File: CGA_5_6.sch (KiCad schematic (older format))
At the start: 5 parts, among them U13 74LS08, U15 74LS00, U20 74LS04, U21 74LS174, U64 74LS164

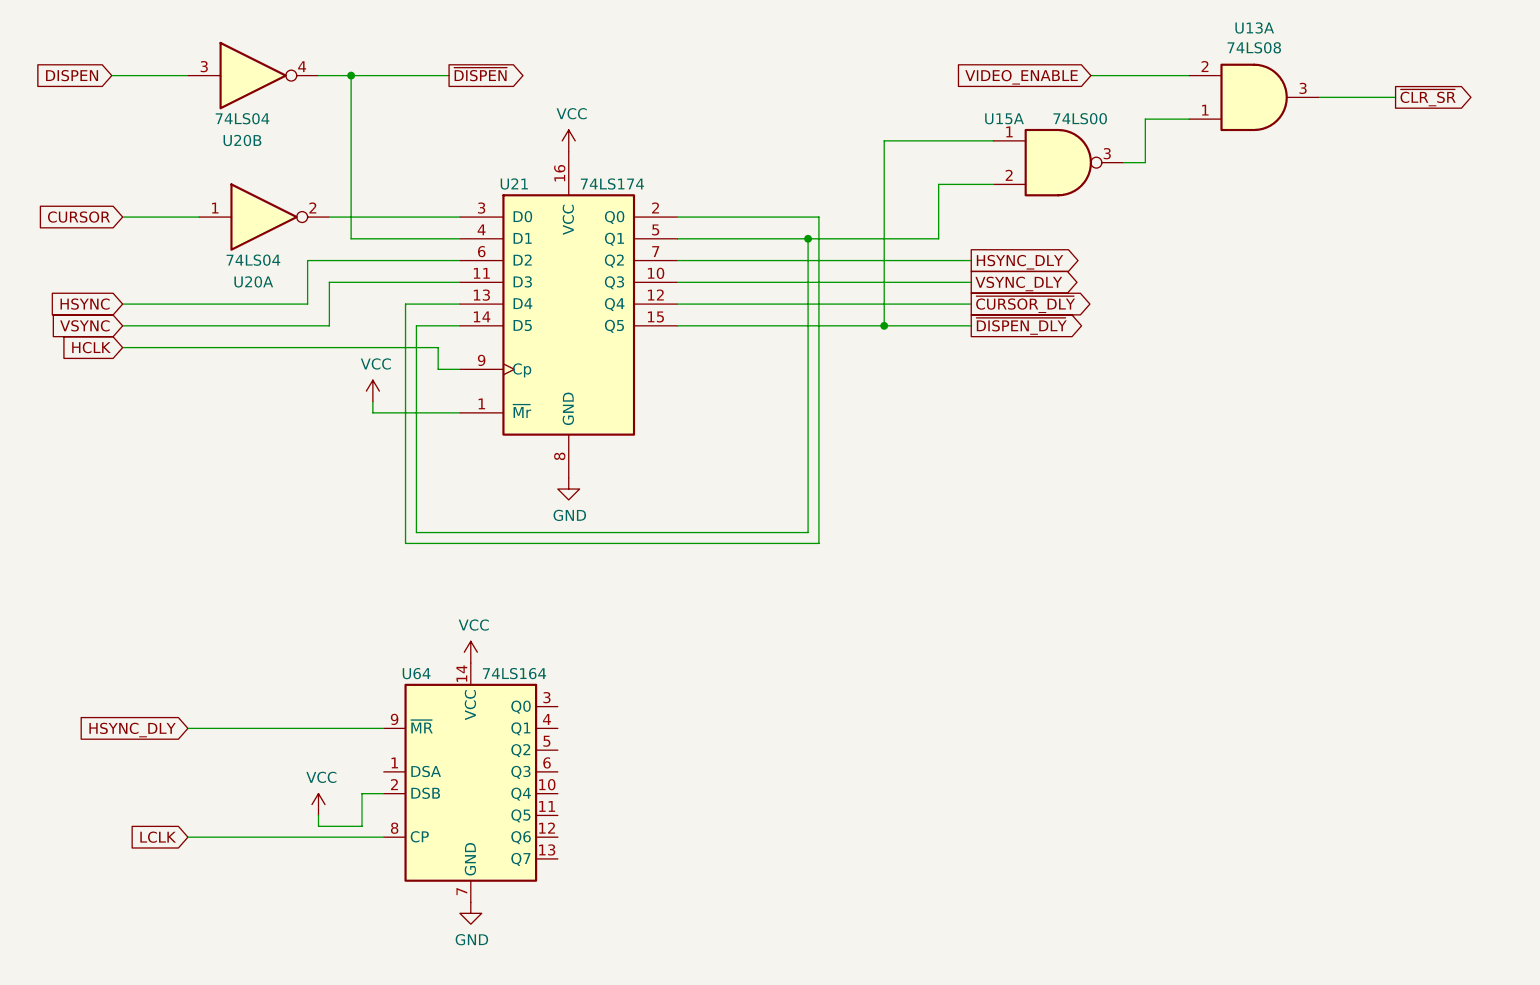
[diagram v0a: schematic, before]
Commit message: More Sheet 5
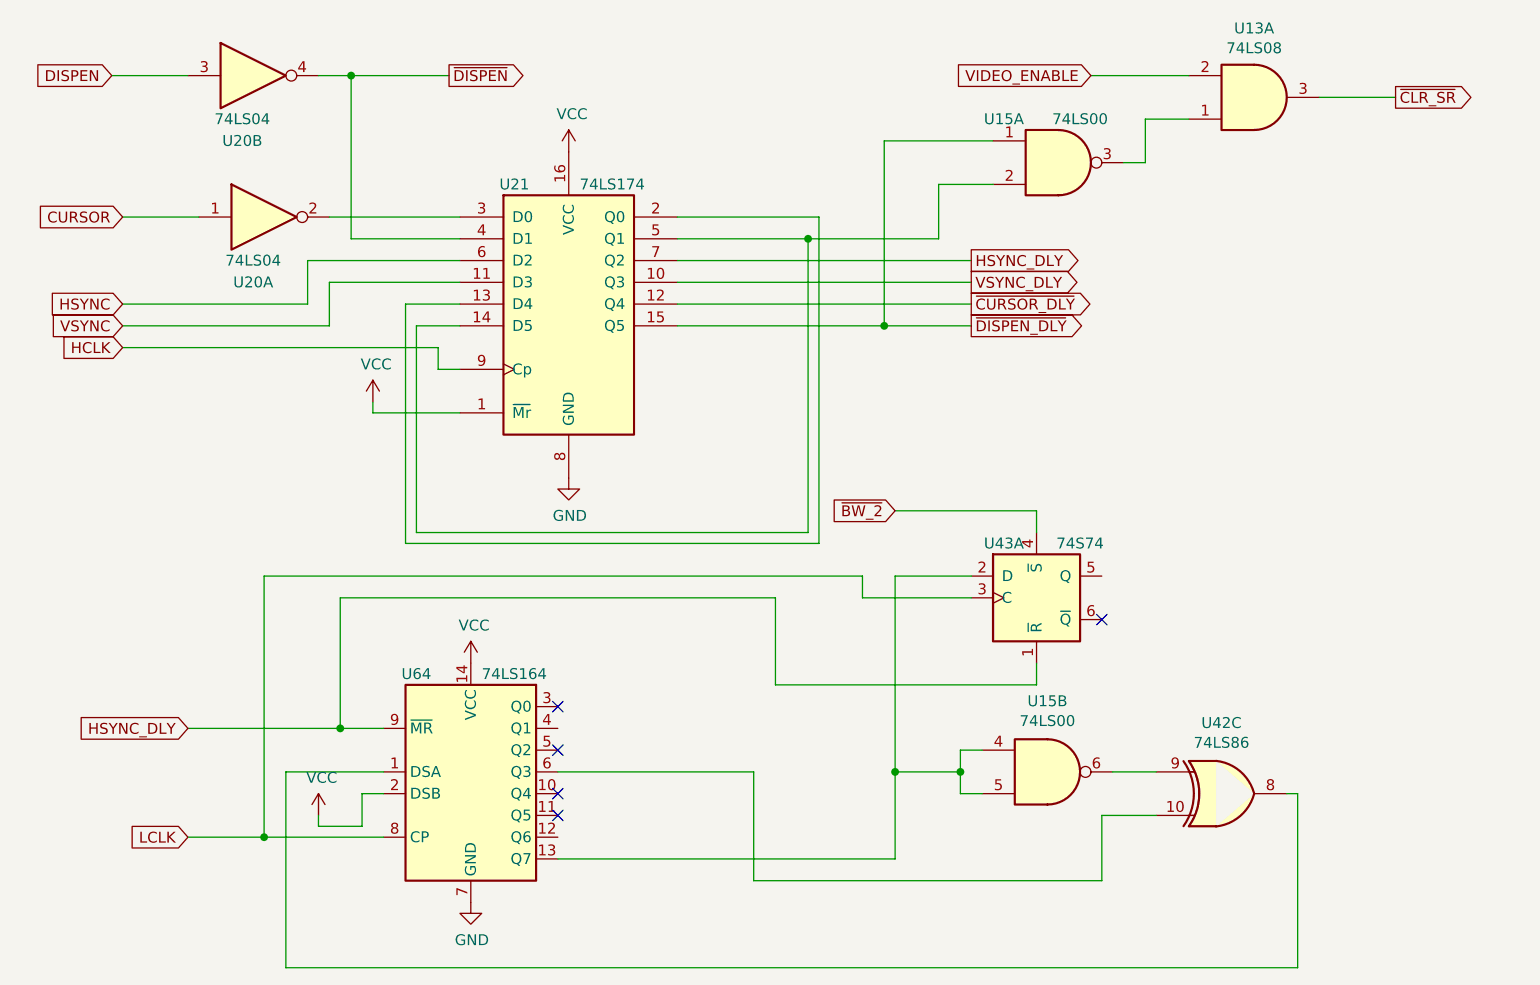
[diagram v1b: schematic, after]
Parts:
- added unit 2 of U15
- added U42: 74LS86, Package_DIP:DIP-14_W7.62mm_LongPads, symbol 74xx:74LS86
- added U43: 74S74, Package_DIP:DIP-14_W7.62mm_LongPads, symbol 74xx:74LS74
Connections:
- net HSYNC_DLY: now also U43.1 (~R)
- net LCLK: now also U43.3 (C)
- net at U64.1 (DSA): now also U42.8
- net at U64.13 (Q7): now also U15.4, U15.5, U43.2 (D)
- net at U64.6 (Q3): now also U42.10
- new net: U15.6, U42.9
- new net ~BW_2: U43.4 (~S)
- no-connect marks 0 -> 5
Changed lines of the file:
@@
 LCLK
 Wire Wire Line
-	2200 4350 1300 4350
+	2200 4350 1650 4350
 Text GLabel 1300 3850 0    50   Input ~ 0
 HSYNC_DLY
 Wire Wire Line
-	2200 3850 1300 3850
+	2200 3850 2000 3850
+$Comp
+L 74xx:74LS74 U43
+U 1 1 63FCF789
+P 5200 3250
+F 0 "U43" H 5050 3500 50  0000 C CNN
+F 1 "74S74" H 5400 3500 50  0000 C CNN
+F 2 "Package_DIP:DIP-14_W7.62mm_LongPads" H 5200 3250 50  0001 C CNN
+F 3 "74xx/74hc_hct74.pdf" H 5200 3250 50  0001 C CNN
+	1    5200 3250
+	1    0    0    -1
+$EndComp
+NoConn ~ 3000 4250
+NoConn ~ 3000 4150
+NoConn ~ 3000 3950
+NoConn ~ 3000 3750
+Wire Wire Line
+	2000 3850 2000 3250
+Wire Wire Line
+	2000 3250 4000 3250
+Wire Wire Line
+	4000 3250 4000 3650
+Wire Wire Line
+	4000 3650 5200 3650
+Wire Wire Line
+	5200 3650 5200 3550
+Connection ~ 2000 3850
+Wire Wire Line
+	2000 3850 1300 3850
+Wire Wire Line
+	3000 4450 4550 4450
+Wire Wire Line
+	4550 4450 4550 4050
+Wire Wire Line
+	4550 3150 4900 3150
+Wire Wire Line
+	1650 4350 1650 3150
+Wire Wire Line
+	1650 3150 4400 3150
+Wire Wire Line
+	4400 3150 4400 3250
+Wire Wire Line
+	4400 3250 4900 3250
+Connection ~ 1650 4350
+Wire Wire Line
+	1650 4350 1300 4350
+Text GLabel 4550 2850 0    50   Input ~ 0
+~BW_2
+Wire Wire Line
+	4550 2850 5200 2850
+Wire Wire Line
+	5200 2850 5200 2950
+NoConn ~ 5500 3350
+$Comp
+L 74xx:74LS00 U?
+U 2 1 63FF0248
+P 5250 4050
+AR Path="/60463C57/63FF0248" Ref="U?"  Part="4"
+AR Path="/60463CF3/63FF0248" Ref="U15"  Part="2"
+F 0 "U15" H 5250 4375 50  0000 C CNN
+F 1 "74LS00" H 5250 4284 50  0000 C CNN
+F 2 "Package_DIP:DIP-14_W7.62mm_LongPads" H 5250 4050 50  0001 C CNN
+F 3 "http://www.ti.com/lit/gpn/sn74ls00" H 5250 4050 50  0001 C CNN
+	2    5250 4050
+	1    0    0    -1
+$EndComp
+Wire Wire Line
+	4950 3950 4850 3950
+Wire Wire Line
+	4850 3950 4850 4050
+Wire Wire Line
+	4850 4150 4950 4150
+Wire Wire Line
+	4850 4050 4550 4050
+Connection ~ 4850 4050
+Wire Wire Line
+	4850 4050 4850 4150
+Connection ~ 4550 4050
+Wire Wire Line
+	4550 4050 4550 3150
+$Comp
+L 74xx:74LS86 U?
+U 3 1 640026CD
+P 6050 4150
+AR Path="/60463C10/640026CD" Ref="U?"  Part="4"
+AR Path="/60463C57/640026CD" Ref="U?"  Part="1"
+AR Path="/60463CF3/640026CD" Ref="U42"  Part="3"
+F 0 "U42" H 6050 4475 50  0000 C CNN
+F 1 "74LS86" H 6050 4384 50  0000 C CNN
+F 2 "Package_DIP:DIP-14_W7.62mm_LongPads" H 6050 4150 50  0001 C CNN
+F 3 "74xx/74ls86.pdf" H 6050 4150 50  0001 C CNN
+	3    6050 4150
+	1    0    0    -1
+$EndComp
+Wire Wire Line
+	5550 4050 5750 4050
+Wire Wire Line
+	3000 4050 3900 4050
+Wire Wire Line
+	3900 4050 3900 4550
+Wire Wire Line
+	3900 4550 5500 4550
+Wire Wire Line
+	5500 4550 5500 4250
+Wire Wire Line
+	5500 4250 5750 4250
+Wire Wire Line
+	6350 4150 6400 4150
+Wire Wire Line
+	6400 4150 6400 4950
+Wire Wire Line
+	6400 4950 1750 4950
+Wire Wire Line
+	1750 4950 1750 4050
+Wire Wire Line
+	1750 4050 2200 4050
 $EndSCHEMATC
